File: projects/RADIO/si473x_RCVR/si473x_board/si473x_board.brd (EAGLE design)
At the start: 75 x 35 mm, 36 parts, among them IC1 SI4730-D60-GUR

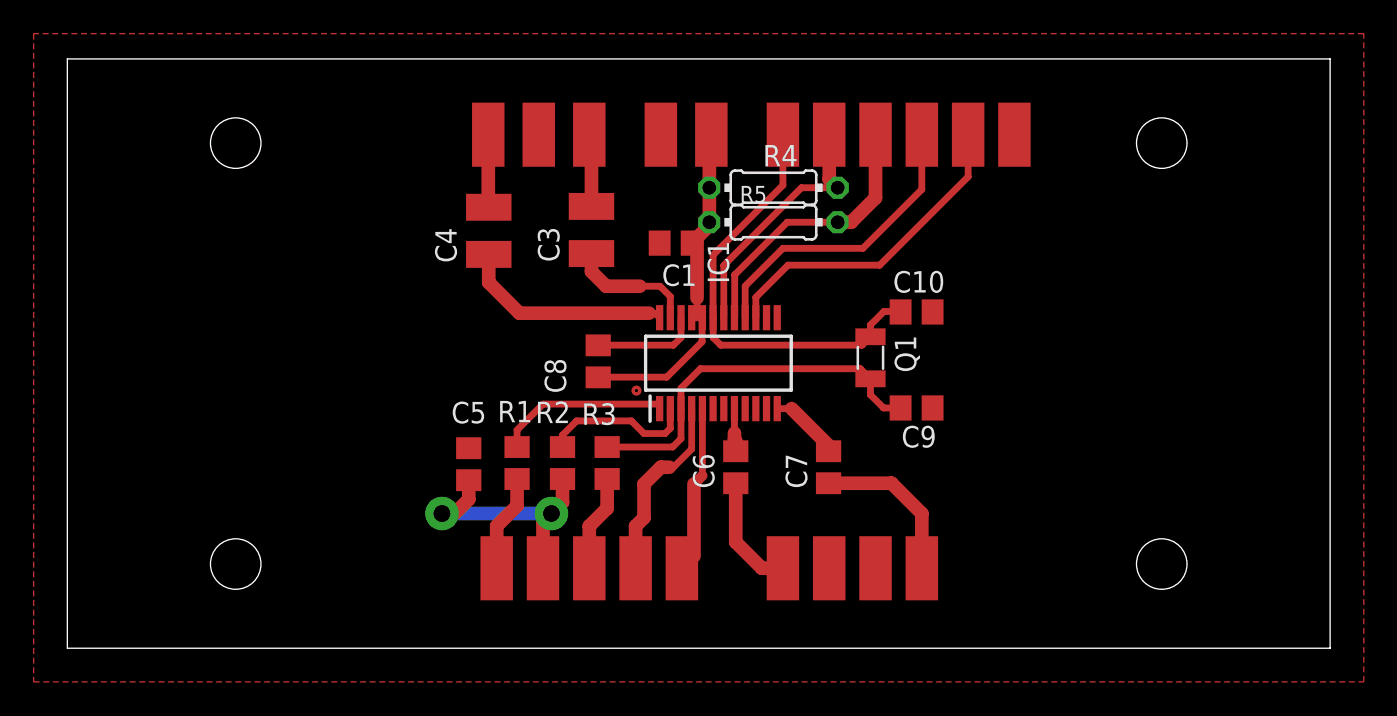
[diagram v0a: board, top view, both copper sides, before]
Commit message: Update
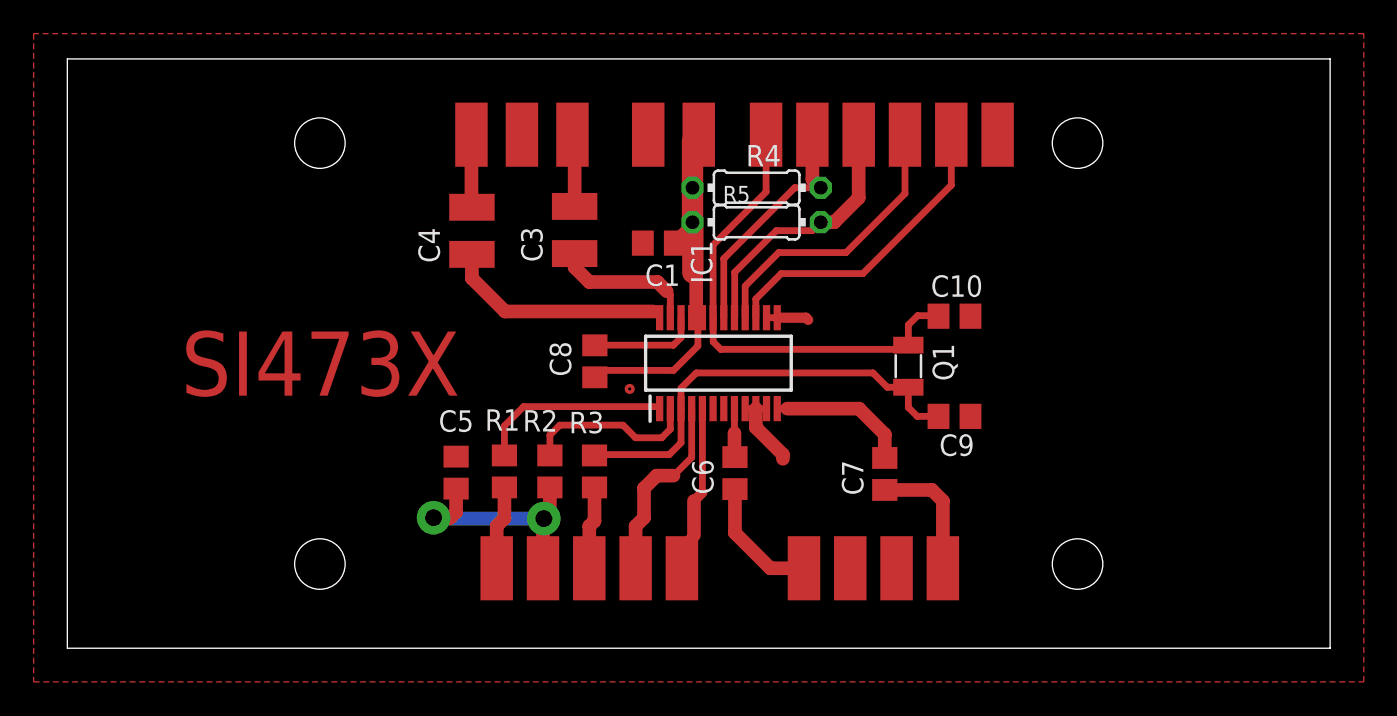
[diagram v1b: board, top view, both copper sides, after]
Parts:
- moved C7 3.36 mm to (48.5, 10.3)
- moved C9 2.30 mm to (52.7, 13.8)
- moved Q1 2.30 mm to (50.0, 16.8)
- moved C10 2.26 mm to (52.7, 19.7)
- moved AMI 1.25 mm to (52.0, 4.75)
- moved FMI 1.25 mm to (43.8, 4.75)
- moved GND 1.25 mm to (46.5, 4.75)
- moved U$8 1.25 mm to (49.2, 4.75)
- moved C1 1.00 mm to (35.1, 24.1)
- moved C3 1.00 mm to (30.1, 24.8)
- moved C4 1.00 mm to (24.0, 24.8)
- moved R4 1.00 mm to (40.9, 27.4)
- moved R5 1.00 mm to (40.9, 25.3)
- moved U$12 1.00 mm to (24.0, 30.5)
- moved U$13 1.00 mm to (27.0, 30.5)
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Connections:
- net N$10 renamed SDA
- net N$11 renamed SCL
- net N$12 renamed SEN
- net N$13 renamed RST
- net N$7 renamed GPOI2
- net N$8 renamed GPIO1
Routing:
- net GND: track 0.00 -> 7.44 mm
- net N$21: track 4.30 -> 8.42 mm
- net GPO3: track 22.6 -> 26.1 mm
- net RCLK: track 26.3 -> 28.7 mm
- net N$22: track 9.54 -> 7.72 mm
- net N$2: track 9.07 -> 10.3 mm
- net N$1: track 10.4 -> 11.6 mm
- net VCC: track 20.8 -> 21.8 mm
- net N$5: track 15.4 -> 14.4 mm
- net SCL: track 16.6 -> 15.6 mm
- net N$14: track 7.62 -> 8.54 mm
- net N$16: track 12.8 -> 13.6 mm
- net SEN: track 18.0 -> 17.1 mm
- net N$6: track 5.74 -> 4.93 mm
- net N$4: track 5.80 -> 4.99 mm
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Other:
- board text added: "SI473X"
